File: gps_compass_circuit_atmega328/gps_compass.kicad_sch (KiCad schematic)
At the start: 31 parts

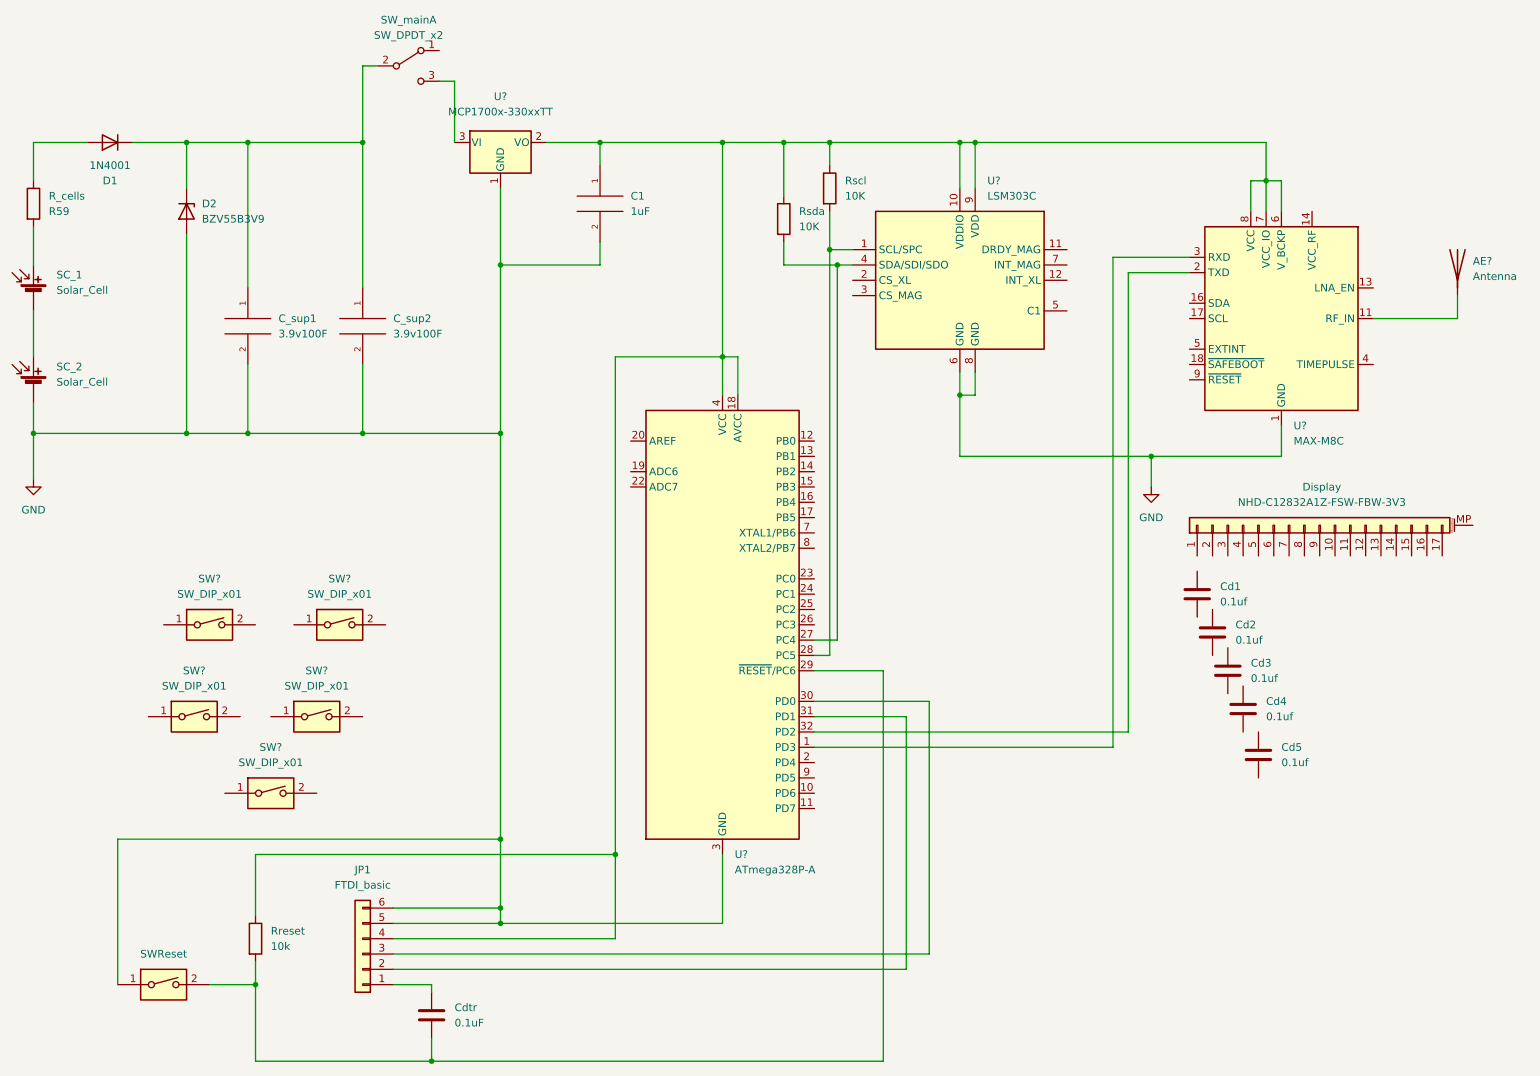
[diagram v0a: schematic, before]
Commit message: Aggiornato circuito
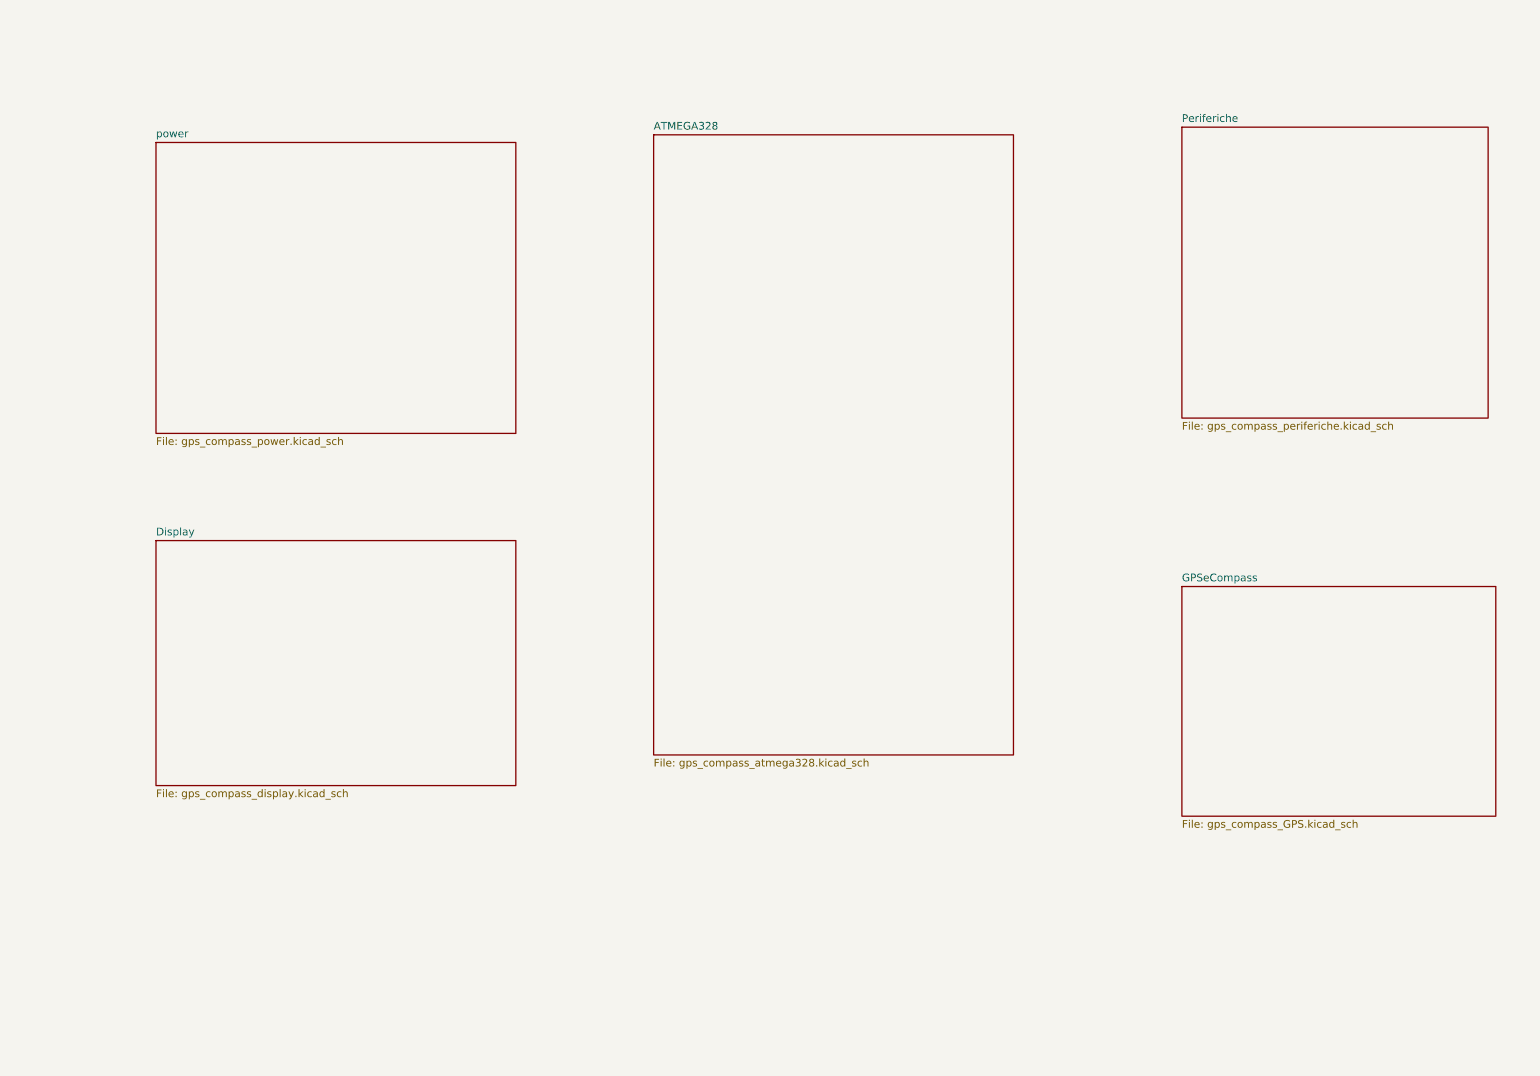
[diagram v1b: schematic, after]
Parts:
- removed AE?: Antenna, symbol Device:Antenna
- removed C1: 1uF, symbol pspice:C
- removed C_sup1, C_sup2: 3.9v100F, symbol pspice:C
- removed Cd1, Cd2, Cd3, Cd4, Cd5: 0.1uf, symbol Device:C
- removed Cdtr: 0.1uF, symbol Device:C
- removed D1: 1N4001, Diode_THT:D_DO-41_SOD81_P10.16mm_Horizontal, symbol Diode:1N4001
- removed D2: BZV55B3V9, Diode_SMD:D_MiniMELF, symbol Diode:BZV55B3V9
- removed Display: NHD-C12832A1Z-FSW-FBW-3V3, symbol Connector_Generic_MountingPin:Conn_01x17_MountingPin
- removed JP1: FTDI_basic, Connector_PinSocket_2.54mm:PinSocket_1x06_P2.54mm_Vertical, symbol Connector_Generic:Conn_01x06
- removed R_cells: R59, symbol Device:R
- removed Rreset: 10k, symbol Device:R
- removed Rscl, Rsda: 10K, symbol Device:R
- removed SC_1, SC_2: Solar_Cell, symbol Device:Solar_Cell
- removed SW? (x5): SW_DIP_x01, symbol Switch:SW_DIP_x01
- removed SWReset: SW_Reset, symbol Switch:SW_DIP_x01
- removed SW_main: SW_DPDT_x2, symbol Switch:SW_DPDT_x2
- removed U?: MCP1700x-330xxTT, Package_TO_SOT_SMD:SOT-23, symbol Regulator_Linear:MCP1700x-330xxTT
- removed U?: MAX-M8C, RF_GPS:ublox_MAX, symbol RF_GPS:MAX-M8C
- removed U?: ATmega328P-A, Package_QFP:TQFP-32_7x7mm_P0.8mm, symbol MCU_Microchip_ATmega:ATmega328P-A
- removed U?: LSM303C, Package_LGA:LGA-12_2x2mm_P0.5mm, symbol Sensor_Motion:LSM303C
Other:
- added sheet ATMEGA328 (gps_compass_atmega328.kicad_sch)
- added sheet Display (gps_compass_display.kicad_sch)
- added sheet GPSeCompass (gps_compass_GPS.kicad_sch)
- added sheet Periferiche (gps_compass_periferiche.kicad_sch)
- added sheet power (gps_compass_power.kicad_sch)
